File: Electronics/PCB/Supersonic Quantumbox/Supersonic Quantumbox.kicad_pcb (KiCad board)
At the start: 2 copper layers, 80 x 150 mm, 76 parts, among them J1 USB_C_Receptacle_USB2.0, J2 Barrel_Jack_Switch, J3 UART, J4 GPIO2, J5 GPIO1, SW1 RESET, SW2 BOOT, SW3 RotaryEncoder_Switch, SW4 SW_DPDT_x2, U1 Input_jack, U2 TL071, U3 PCM1808PWR, U4 AZ1117-5.0, U5 ESP32-S2-WROVER-I, U6 AZ1117-3.3, U7 PCM5100, U8 Output_jack

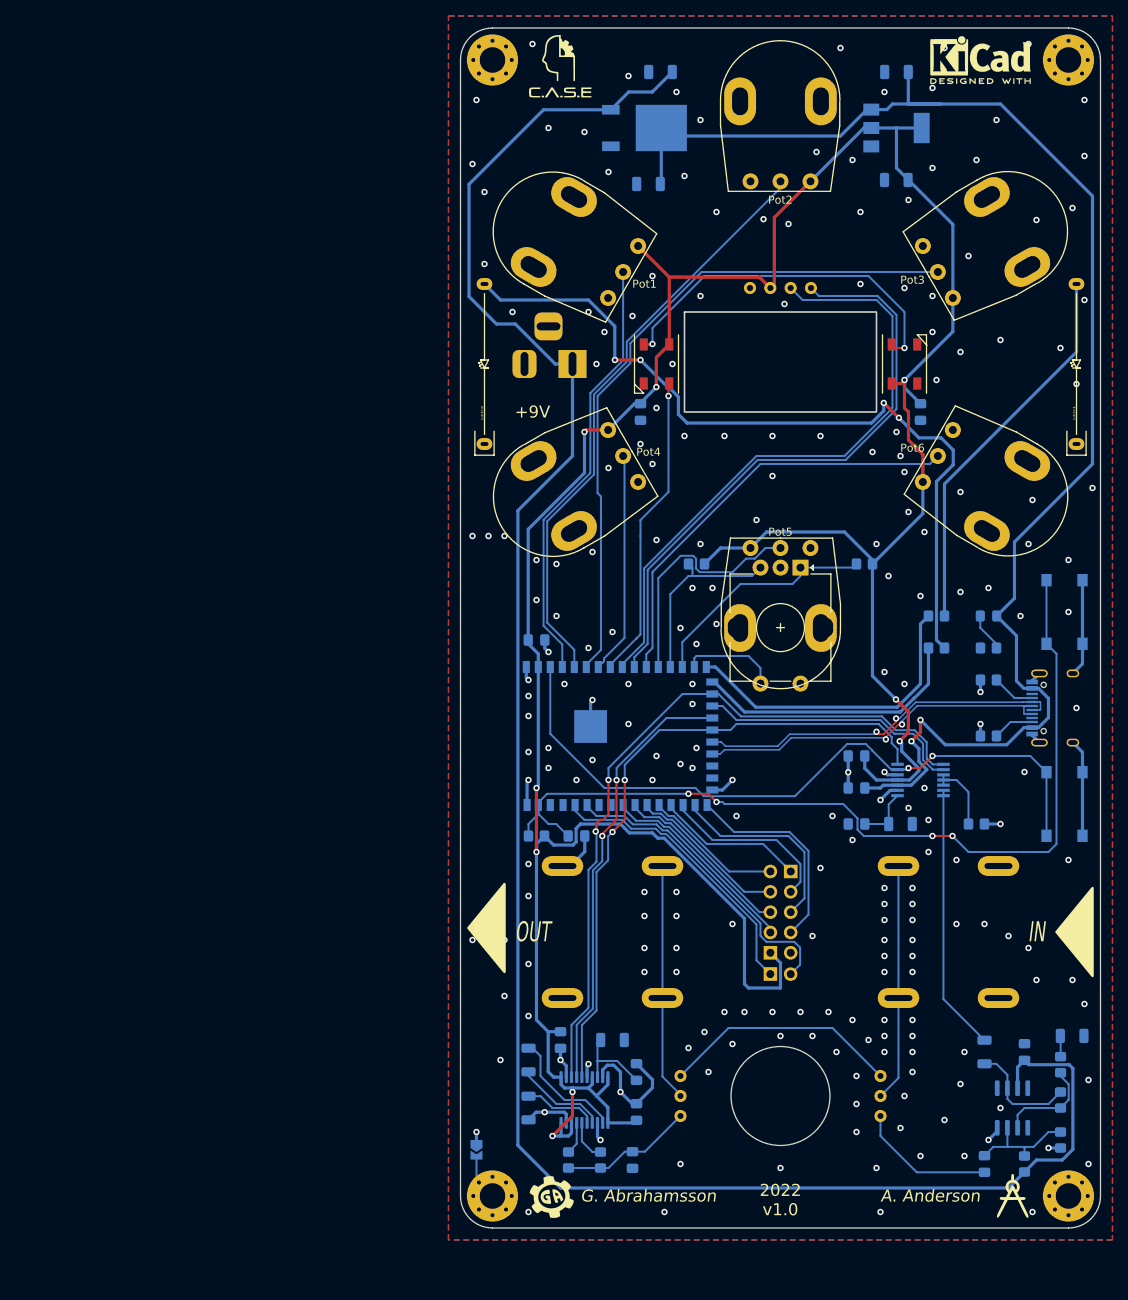
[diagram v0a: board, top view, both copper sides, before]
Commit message: Add Gerbs
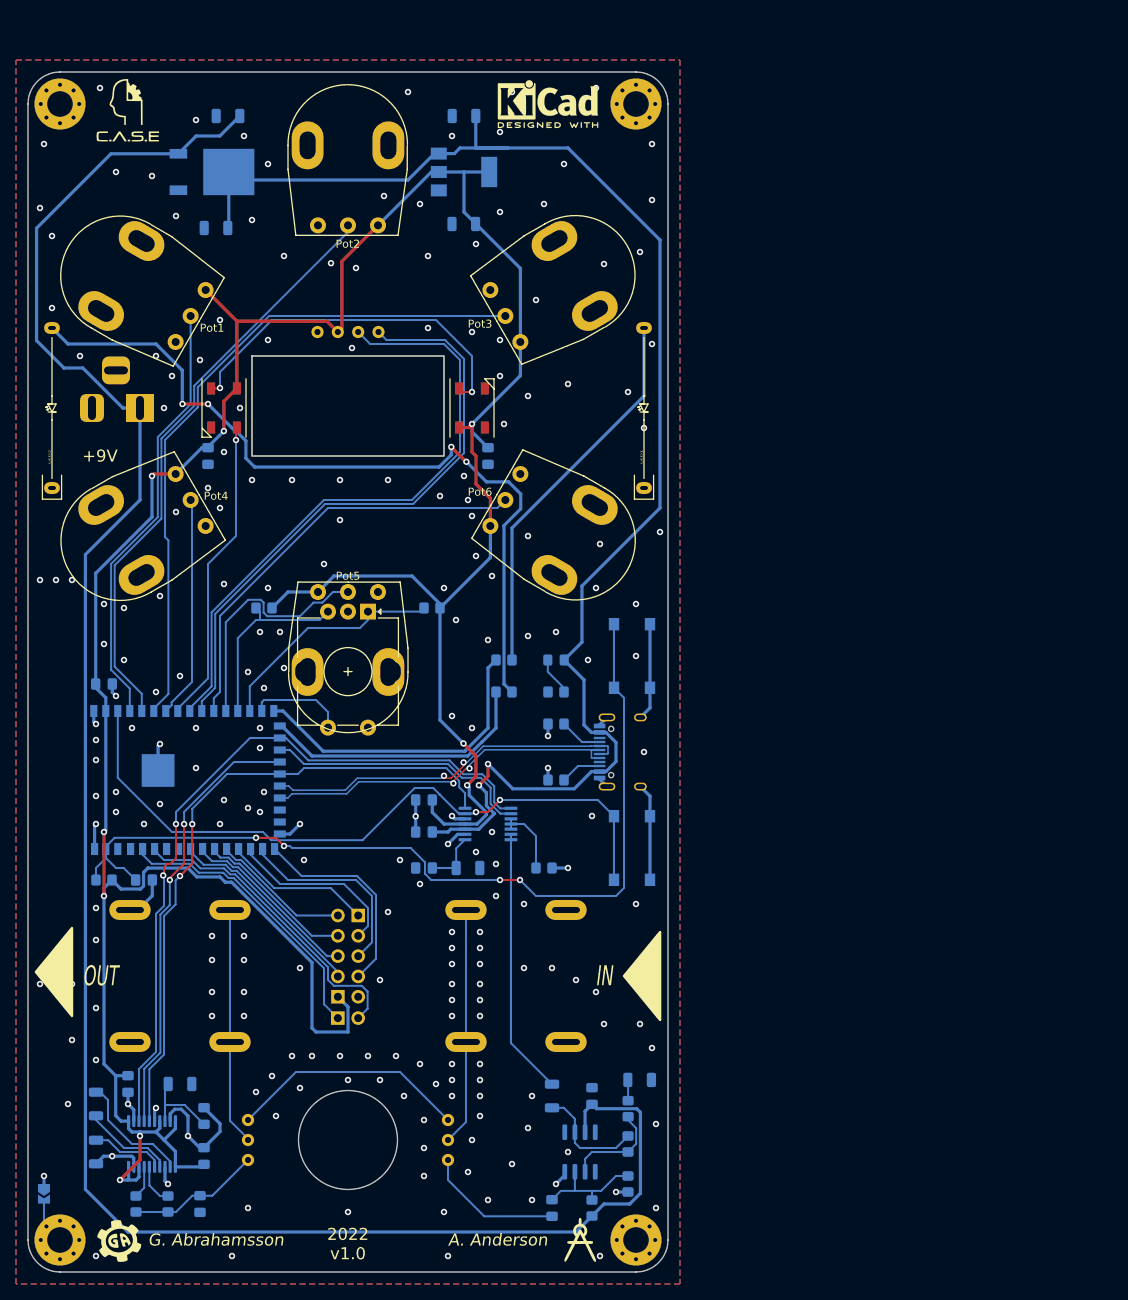
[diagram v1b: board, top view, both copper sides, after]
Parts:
- moved C1 54.3 mm to (154.4, 165.0)
- moved C20 54.3 mm to (159.4, 151.0)
- moved C21 54.3 mm to (143.9, 122.5)
- moved C23 54.3 mm to (146.4, 71.0)
- moved C3 54.3 mm to (154.4, 151.0)
- moved C4 54.3 mm to (138.4, 118.0)
- moved C5 54.3 mm to (138.4, 114.0)
- moved C6 54.3 mm to (138.4, 122.5)
- moved C9 54.3 mm to (143.4, 28.5)
- moved D2 54.3 mm to (144.4, 65.0)
- moved D4 54.3 mm to (165.9, 65.0)
- moved D5 54.3 mm to (154.9, 96.5)
- moved G*** 54.3 mm to (157.9, 169.0)
- moved H2 54.3 mm to (164.9, 169.0)
- moved H4 54.3 mm to (164.9, 27.0)
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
